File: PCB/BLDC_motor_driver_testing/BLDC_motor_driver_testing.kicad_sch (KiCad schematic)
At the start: 4 parts

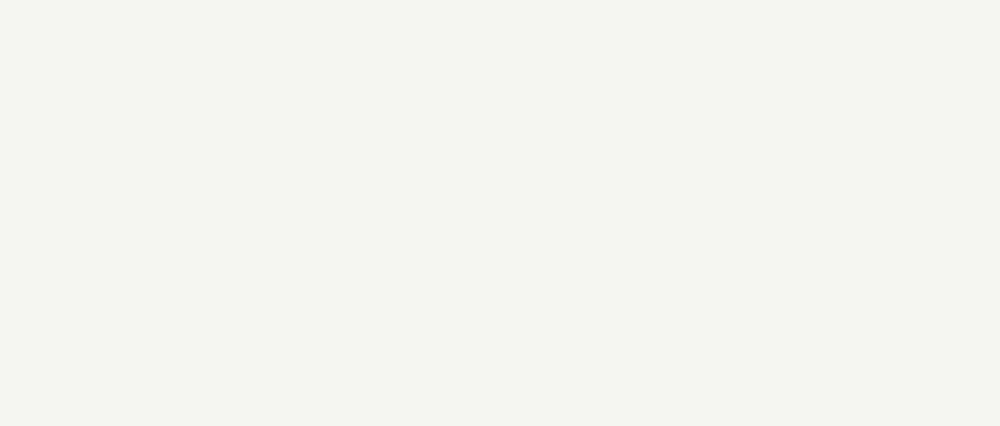
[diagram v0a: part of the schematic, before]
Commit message: PCB progress...
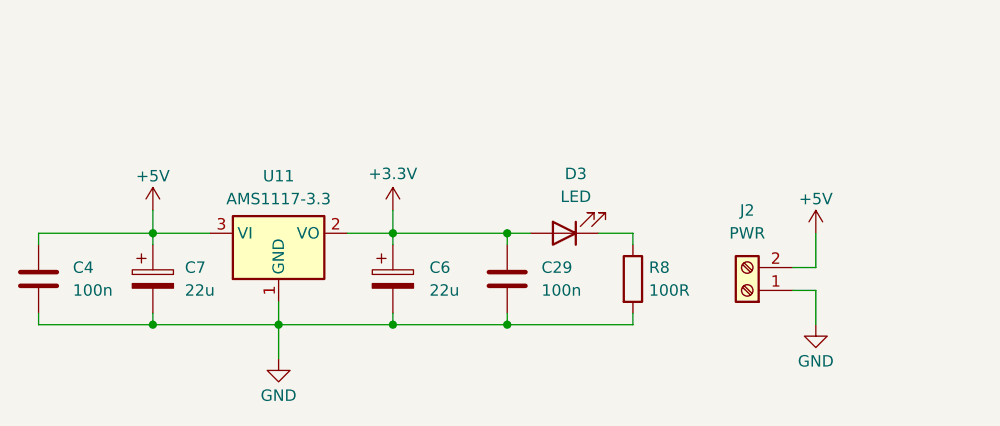
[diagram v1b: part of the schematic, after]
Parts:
- added C29, C4: 100n, Capacitor_SMD:C_0504_1310Metric, symbol Device:C
- added C6, C7: 22u, symbol Device:C_Polarized
- added D3: LED, LED_SMD:LED_0402_1005Metric, symbol Device:LED
- added J2: PWR, TerminalBlock:TerminalBlock_Xinya_XY308-2.54-2P_1x02_P2.54mm_Horizontal, symbol Connector:Screw_Terminal_01x02
- added R8: 100R, Resistor_SMD:R_0402_1005Metric, symbol Device:R
- added U11: AMS1117-3.3, Package_TO_SOT_SMD:SOT-223-3_TabPin2, symbol Regulator_Linear:AMS1117-3.3
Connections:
- new net: D3.1 (K), R8.1
- new net +3.3V: C29.1, C6.1, D3.2 (A), U11.2 (VO)
- new net +5V: C4.1, C7.1, J2.2 (Pin_2), U11.3 (VI)
- new net GND: C29.2, C4.2, C6.2, C7.2, J2.1 (Pin_1), R8.2, U11.1 (GND)

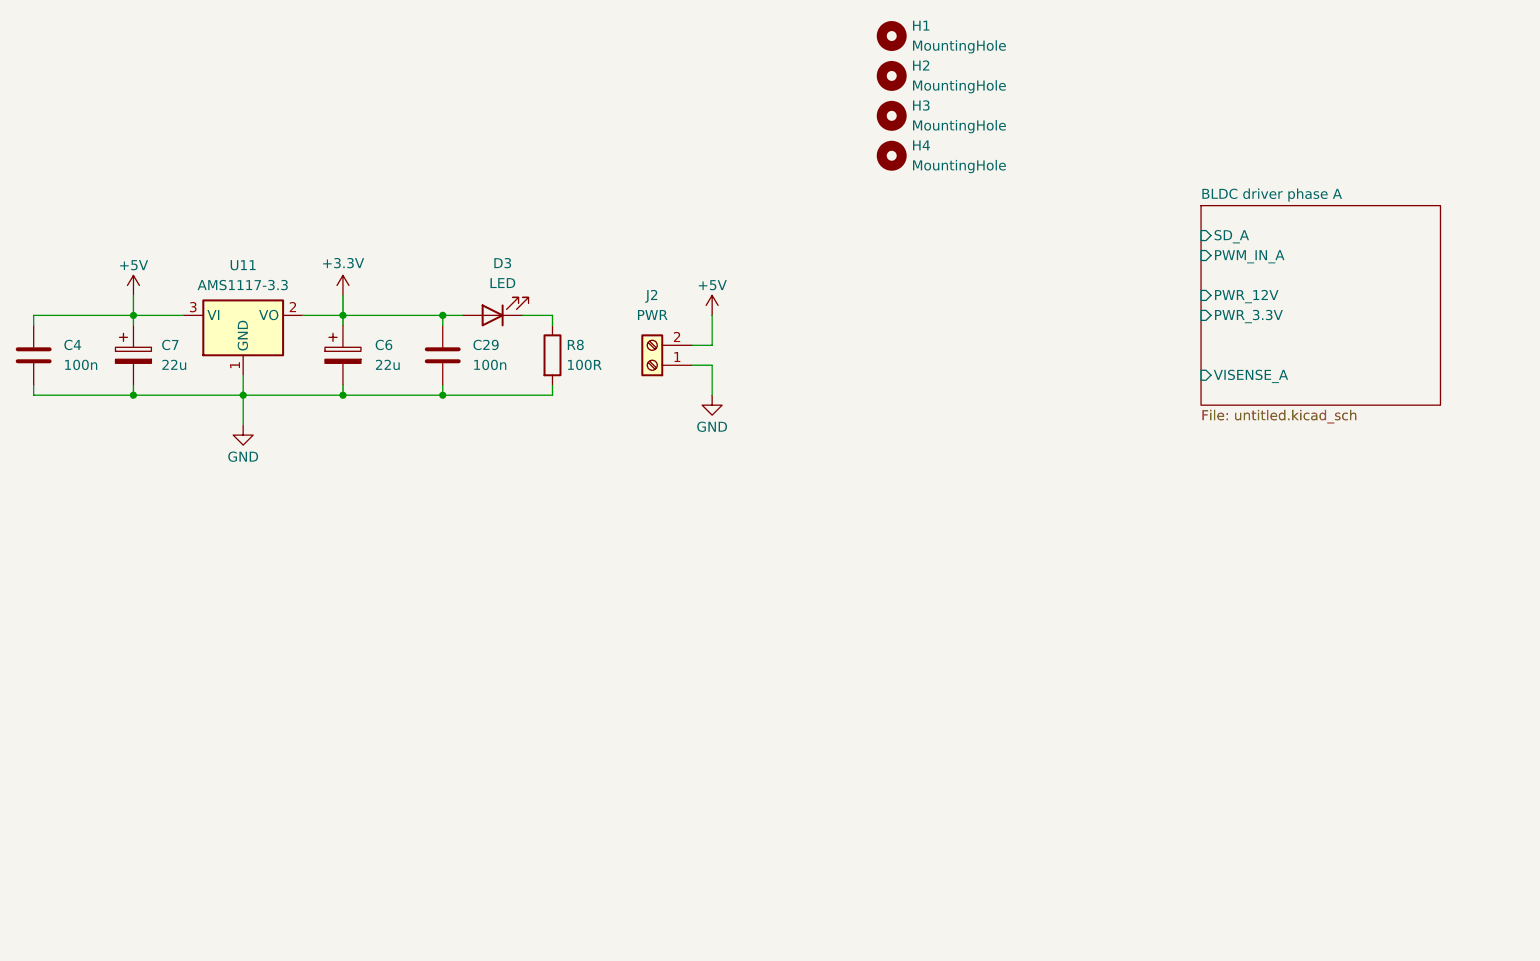
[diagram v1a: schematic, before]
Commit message: PCB progress...
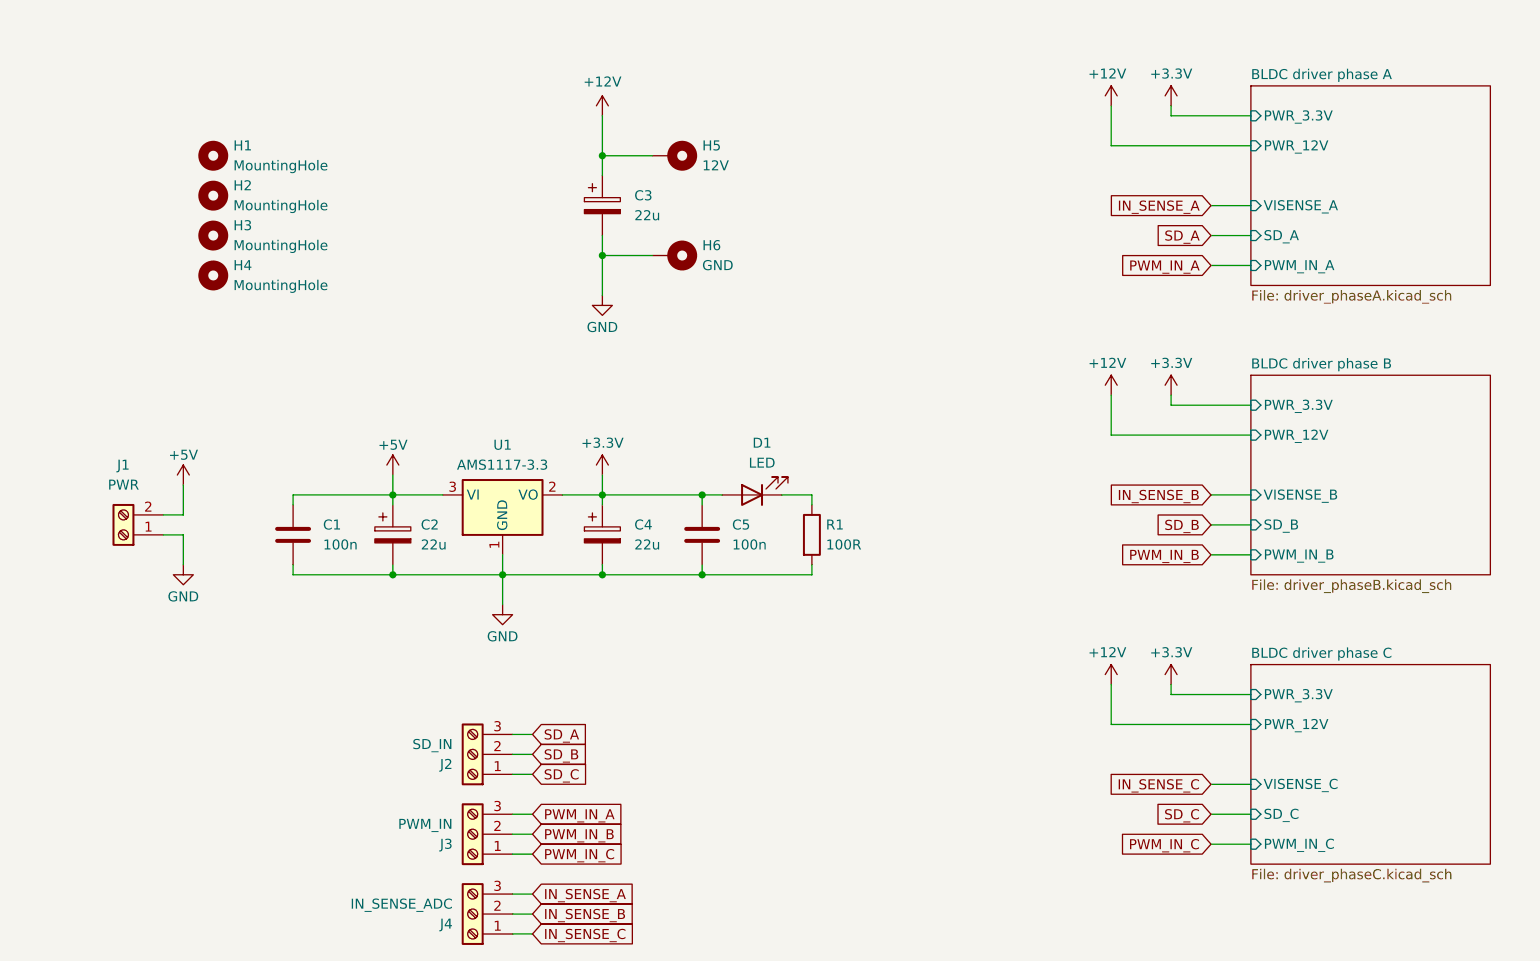
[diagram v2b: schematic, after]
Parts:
- added C3: 22u, Capacitor_SMD:C_0805_2012Metric_Pad1.18x1.45mm_HandSolder, symbol Device:C_Polarized
- added H5: 12V, MountingHole:MountingHole_2.2mm_M2_Pad_TopBottom, symbol Mechanical:MountingHole_Pad
- added H6: GND, MountingHole:MountingHole_2.2mm_M2_Pad_TopBottom, symbol Mechanical:MountingHole_Pad
- added J2: SD_IN, TerminalBlock:TerminalBlock_Xinya_XY308-2.54-3P_1x03_P2.54mm_Horizontal, symbol Connector:Screw_Terminal_01x03
- added J3: PWM_IN, TerminalBlock:TerminalBlock_Xinya_XY308-2.54-3P_1x03_P2.54mm_Horizontal, symbol Connector:Screw_Terminal_01x03
- added J4: IN_SENSE_ADC, TerminalBlock:TerminalBlock_Xinya_XY308-2.54-3P_1x03_P2.54mm_Horizontal, symbol Connector:Screw_Terminal_01x03
- C1: renamed from C4; footprint Capacitor_SMD:C_0504_1310Metric -> Capacitor_SMD:C_0805_2012Metric_Pad1.18x1.45mm_HandSolder
- C2: renamed from C7; footprint (none) -> Capacitor_SMD:C_0805_2012Metric_Pad1.18x1.45mm_HandSolder
- C4: renamed from C6; footprint (none) -> Capacitor_SMD:C_0805_2012Metric_Pad1.18x1.45mm_HandSolder
- C5: renamed from C29; footprint Capacitor_SMD:C_0504_1310Metric -> Capacitor_SMD:C_0805_2012Metric_Pad1.18x1.45mm_HandSolder
- D1: renamed from D3; footprint LED_SMD:LED_0402_1005Metric -> LED_SMD:LED_0805_2012Metric_Pad1.15x1.40mm_HandSolder
- R1: renamed from R8; footprint Resistor_SMD:R_0402_1005Metric -> Resistor_SMD:R_0805_2012Metric_Pad1.20x1.40mm_HandSolder
- renumbered J2 to J1, U11 to U1
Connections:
- net GND: now also C3.2, H6.1
- new net +12V: C3.1, H5.1
- new net IN_SENSE_A: J4.3 (Pin_3)
- new net IN_SENSE_B: J4.2 (Pin_2)
- new net IN_SENSE_C: J4.1 (Pin_1)
- new net PWM_IN_A: J3.3 (Pin_3)
- new net PWM_IN_B: J3.2 (Pin_2)
- new net PWM_IN_C: J3.1 (Pin_1)
- new net SD_A: J2.3 (Pin_3)
- new net SD_B: J2.2 (Pin_2)
- new net SD_C: J2.1 (Pin_1)
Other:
- added sheet BLDC driver phase B (driver_phaseB.kicad_sch)
- added sheet BLDC driver phase C (driver_phaseC.kicad_sch)
- sheet BLDC driver phase A: file untitled.kicad_sch -> driver_phaseA.kicad_sch
- moved on the sheet: C1, C2, C4, C5, D1, H1, H2, H3, H4, J1, R1, U1
